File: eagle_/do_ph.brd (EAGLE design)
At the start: 80.3 x 73.6 mm, 26 parts, among them IC1 MEGA8-P, Q1 8Mhz

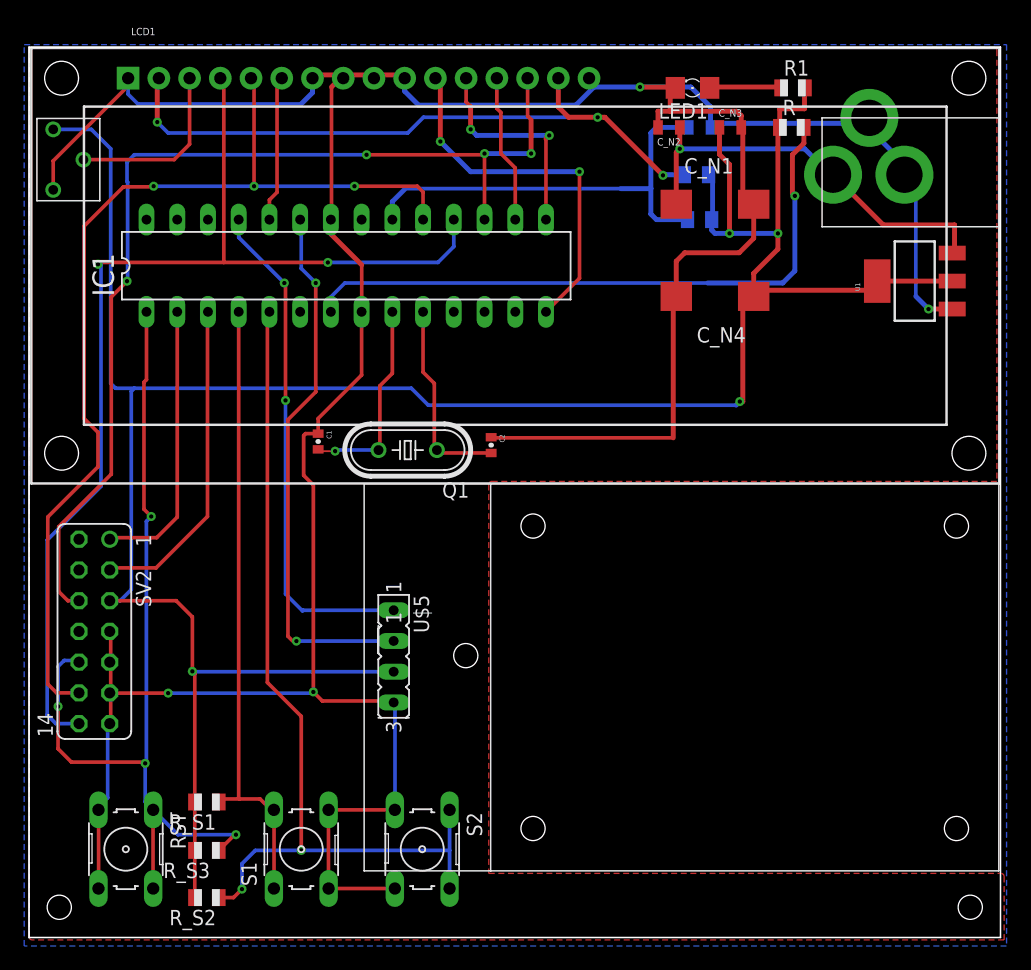
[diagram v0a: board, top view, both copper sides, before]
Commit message: update mạch in
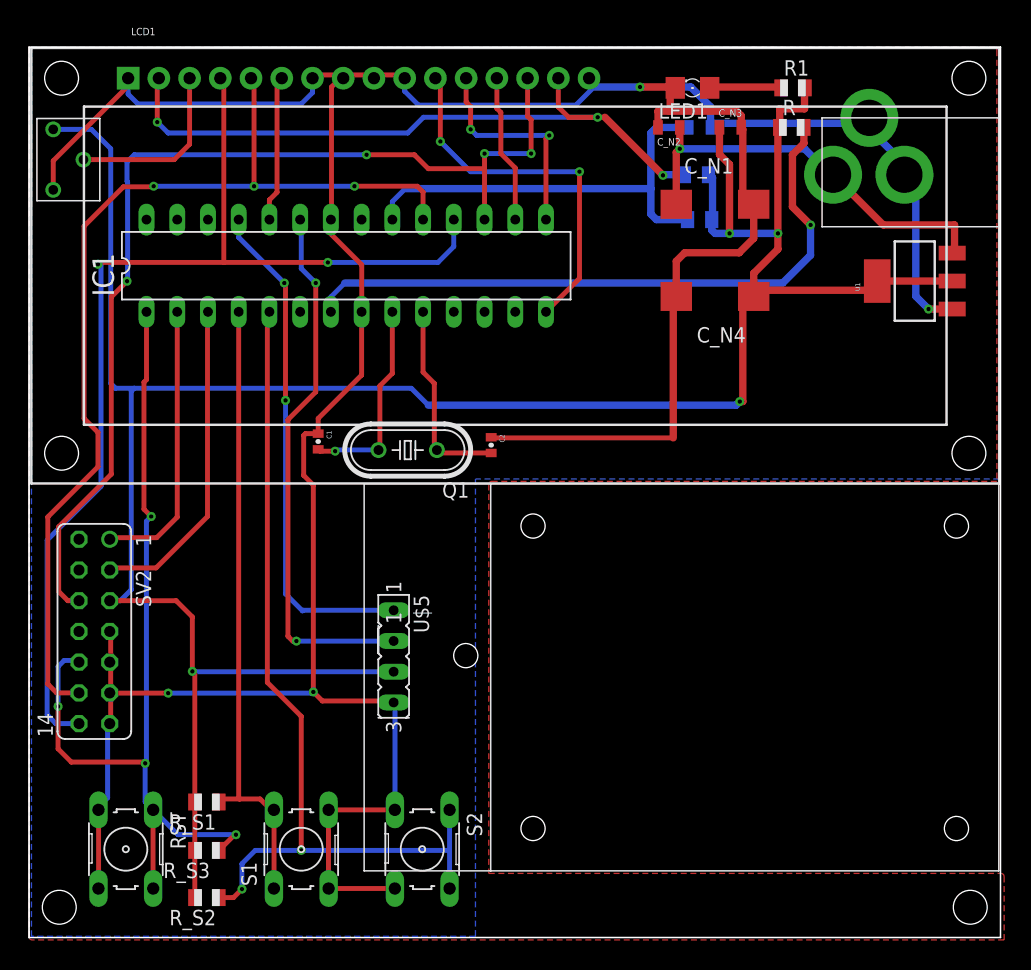
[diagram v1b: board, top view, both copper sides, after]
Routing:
- net N$11: track 52.8 -> 53.9 mm
- net D7: track 85.4 -> 86.1 mm
